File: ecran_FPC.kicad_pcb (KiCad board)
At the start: 4 copper layers, 43 x 43 mm, 24 parts, among them J1 MEC1-110-02-F-D-A, J2 MEC1-110-02-F-D-A, J3 1-2328724-5, SW1 PEC11L-4220K-S0015

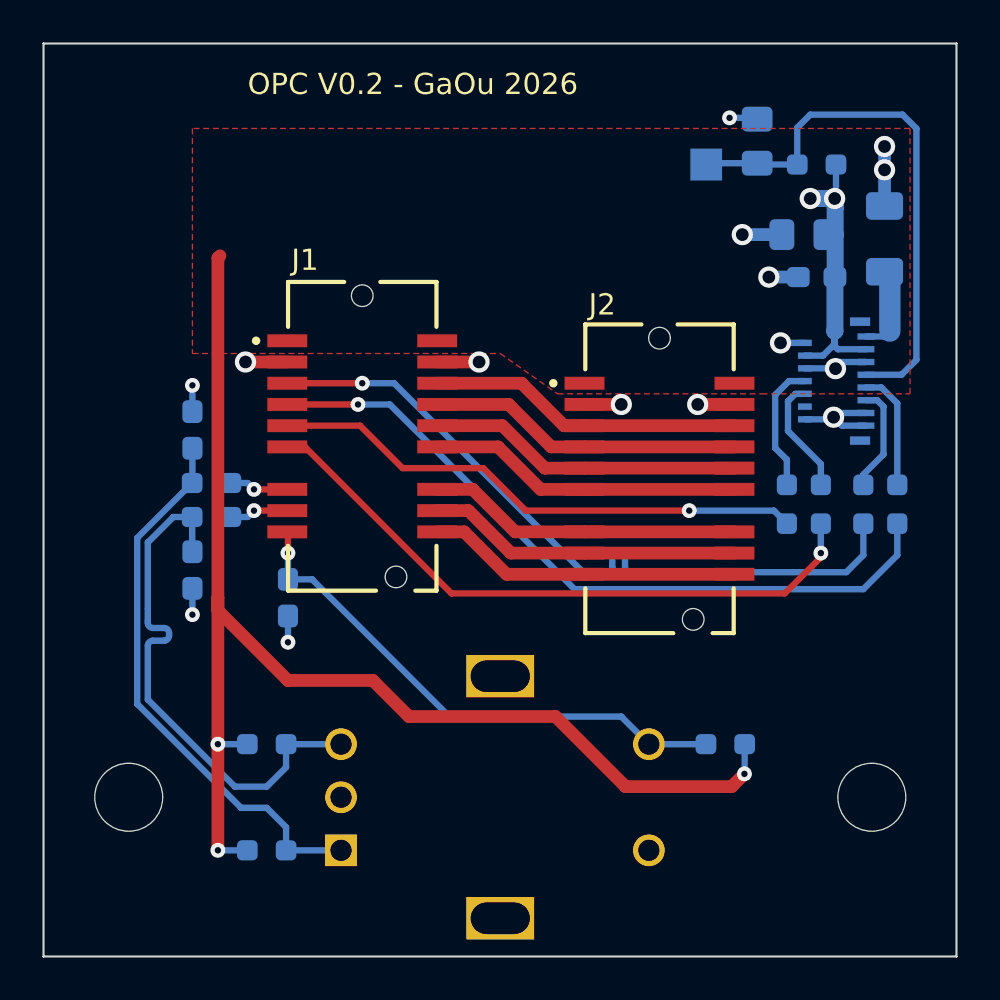
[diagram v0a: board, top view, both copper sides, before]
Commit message: pre prod
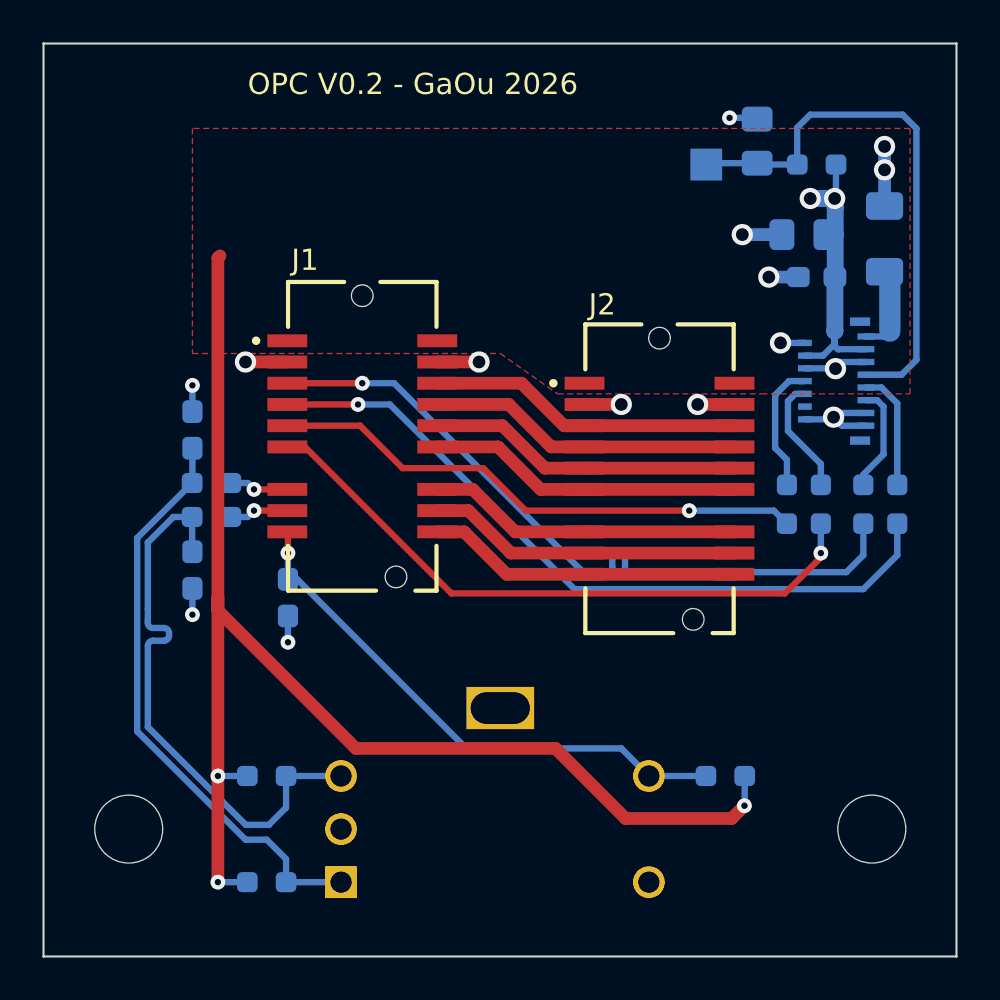
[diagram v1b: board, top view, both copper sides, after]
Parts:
- SW1: value PEC11L-4220K-S0015 -> PEC11L-4220F-S0015
- moved H1 1.50 mm to (104.0, 137.0)
- moved H2 1.50 mm to (139.0, 137.0)
- moved R10 1.50 mm to (110.5, 134.5)
- moved R11 1.50 mm to (110.5, 139.5)
- moved R9 1.50 mm to (132.1, 134.5)
- moved SW1 1.50 mm to (121.5, 137.0)
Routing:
- net +3.3V: track 77.6 -> 79.7 mm
- net Net-(C5-Pad2): track 25.4 -> 27.3 mm
- net Net-(C4-Pad2): track 26.4 -> 27.6 mm
- net /ROTENC_SW: track 25.2 -> 25.8 mm
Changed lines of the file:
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@@
 	(footprint "MountingHole:MountingHole_3.2mm_M3_DIN965"
 		(layer "F.Cu")
-		(at 104 135.5)
+		(at 104 137)
 		(descr "Mounting Hole 3.2mm, M3, no annular, generated by kicad-footprint-generator mountinghole.py")
 		(tags "mountinghole M3 DIN965")
@@
 	(footprint "MountingHole:MountingHole_3.2mm_M3_DIN965"
 		(layer "F.Cu")
-		(at 139 135.5)
+		(at 139 137)
 		(descr "Mounting Hole 3.2mm, M3, no annular, generated by kicad-footprint-generator mountinghole.py")
 		(tags "mountinghole M3 DIN965")
@@
 	(footprint "OPC:PEC11L4220KS0015"
 		(layer "B.Cu")
-		(at 121.5 135.5 90)
+		(at 121.5 137 90)
 		(descr "PEC11L-4220K-S0015-2")
 		(tags "Undefined or Miscellaneous")
 		(property "Reference" "SW1"
-			(at 7.9 0 180)
+			(at 7.9 0 0)
 			(layer "B.SilkS")
 			(effects
@@
 			)
 		)
-		(property "Value" "PEC11L-4220K-S0015"
-			(at 2.5 7.25 90)
+		(property "Value" "PEC11L-4220F-S0015"
+			(at 2.5 7.25 270)
 			(layer "B.SilkS")
 			(hide yes)
@@
 		)
 		(property "Datasheet" ""
-			(at 0 0 90)
+			(at 0 0 270)
 			(layer "B.Fab")
 			(hide yes)
@@
 		)
 		(property "Description" "Rotary encoder, dual channel, incremental quadrate outputs, with switch and MP Pin"
-			(at 0 0 90)
+			(at 0 0 270)
 			(layer "B.Fab")
 			(hide yes)
@@
 			)
 		)
-		(property "MPN" "PEC11L-4220K-S0015 "
+		(property "MPN" "PEC11L-4220F-S0015 "
 			(at 0 0 90)
 			(unlocked yes)
@@
 			)
 		)
-		(property "px_1" "2.13"
+		(property "px_1" "2.35"
 			(at 0 0 90)
 			(unlocked yes)
@@
 			)
 		)
-		(property "px_10" "1.78"
+		(property "px_10" "2.02"
 			(at 0 0 90)
 			(unlocked yes)
@@
 		)
 		(fp_text user "${REFERENCE}"
-			(at 0 -11 90)
+			(at 0 -11 270)
 			(layer "B.Fab")
 			(effects
@@
 		)
 		(pad "MP" thru_hole rect
-			(at -5.7 0)
-			(size 3.2 2)
-			(drill oval 2.8 1.5)
-			(layers "*.Cu" "*.Mask")
-			(remove_unused_layers no)
-			(net "unconnected-(SW1-PadMP)")
-			(pinfunction "MP_MP")
-			(pintype "passive")
-		)
-		(pad "MP" thru_hole rect
 			(at 5.7 0)
 			(size 3.2 2)
@@
 	(footprint "Resistor_SMD:R_0603_1608Metric_Pad0.98x0.95mm_HandSolder"
 		(layer "B.Cu")
-		(at 132.1 133)
+		(at 132.1 134.5)
 		(descr "Resistor SMD 0603 (1608 Metric), square (rectangular) end terminal, IPC-7351 nominal with elongated pad for handsoldering. (Body size source: IPC-SM-782 page 72, https://www.pcb-3d.com/wordpress/wp-content/uploads/ipc-sm-782a_amendment_1_and_2.pdf)")
 		(tags "resistor handsolder")
@@
 	(footprint "Resistor_SMD:R_0603_1608Metric_Pad0.98x0.95mm_HandSolder"
 		(layer "B.Cu")
-		(at 110.5 133)
+		(at 110.5 134.5)
 		(descr "Resistor SMD 0603 (1608 Metric), square (rectangular) end terminal, IPC-7351 nominal with elongated pad for handsoldering. (Body size source: IPC-SM-782 page 72, https://www.pcb-3d.com/wordpress/wp-content/uploads/ipc-sm-782a_amendment_1_and_2.pdf)")
 		(tags "resistor handsolder")
@@
 	(footprint "Resistor_SMD:R_0603_1608Metric_Pad0.98x0.95mm_HandSolder"
 		(layer "B.Cu")
-		(at 110.5 138)
+		(at 110.5 139.5)
 		(descr "Resistor SMD 0603 (1608 Metric), square (rectangular) end terminal, IPC-7351 nominal with elongated pad for handsoldering. (Body size source: IPC-SM-782 page 72, https://www.pcb-3d.com/wordpress/wp-content/uploads/ipc-sm-782a_amendment_1_and_2.pdf)")
 		(tags "resistor handsolder")
@@
 	)
 	(segment
-		(start 117.2 131.7)
-		(end 124.1 131.7)
+		(start 132.4 136.5)
+		(end 133 135.9)
 		(width 0.6)
 		(layer "F.Cu")
@@
 	)
 	(segment
-		(start 127.4 135)
-		(end 132.4 135)
+		(start 108.2 126.7)
+		(end 114.7 133.2)
 		(width 0.6)
 		(layer "F.Cu")
@@
 	)
 	(segment
-		(start 108.2 126.1)
-		(end 108.2 126.7)
+		(start 124.1 133.2)
+		(end 127.4 136.5)
 		(width 0.6)
 		(layer "F.Cu")
@@
 	)
 	(segment
-		(start 111.5 130)
-		(end 115.5 130)
+		(start 114.7 133.2)
+		(end 124.1 133.2)
 		(width 0.6)
 		(layer "F.Cu")
@@
 	)
 	(segment
-		(start 108.2 133)
-		(end 108.2 126.1)
+		(start 127.4 136.5)
+		(end 132.4 136.5)
 		(width 0.6)
 		(layer "F.Cu")
@@
 	)
 	(segment
-		(start 115.5 130)
-		(end 117.2 131.7)
-		(width 0.6)
-		(layer "F.Cu")
-		(net "+3.3V")
-	)
-	(segment
-		(start 132.4 135)
-		(end 133 134.4)
-		(width 0.6)
-		(layer "F.Cu")
-		(net "+3.3V")
-	)
-	(segment
 		(start 108.3 110)
 		(end 108.2 110.1)
@@
 	)
 	(segment
-		(start 124.1 131.7)
-		(end 127.4 135)
+		(start 108.2 139.5)
+		(end 108.2 134.5)
 		(width 0.6)
 		(layer "F.Cu")
@@
 	)
 	(segment
-		(start 108.2 138)
-		(end 108.2 133)
+		(start 108.2 126.1)
+		(end 108.2 126.7)
 		(width 0.6)
 		(layer "F.Cu")
@@
 	)
 	(segment
-		(start 108.2 126.7)
-		(end 111.5 130)
+		(start 108.2 134.5)
+		(end 108.2 126.1)
 		(width 0.6)
 		(layer "F.Cu")
@@
 	)
 	(via
-		(at 108.2 138)
+		(at 108.2 139.5)
 		(size 0.7)
 		(drill 0.3)
@@
 	)
 	(via
-		(at 133 134.4)
+		(at 133 135.9)
 		(size 0.7)
 		(drill 0.3)
@@
 	)
 	(via
-		(at 108.2 133)
+		(at 108.2 134.5)
 		(size 0.7)
 		(drill 0.3)
@@
 	)
 	(segment
-		(start 109.5875 133)
-		(end 108.2 133)
+		(start 109.5875 134.5)
+		(end 108.2 134.5)
 		(width 0.3)
 		(layer "B.Cu")
@@
 	)
 	(segment
-		(start 133.0125 133)
-		(end 133.0125 134.3875)
+		(start 133.0125 134.5)
+		(end 133.0125 135.8875)
 		(width 0.3)
 		(layer "B.Cu")
@@
 	)
 	(segment
-		(start 109.5875 138)
-		(end 108.2 138)
+		(start 109.5875 139.5)
+		(end 108.2 139.5)
 		(width 0.3)
 		(layer "B.Cu")
@@
 	)
 	(segment
-		(start 133.0125 134.3875)
-		(end 133 134.4)
+		(start 133.0125 135.8875)
+		(end 133 135.9)
 		(width 0.3)
 		(layer "B.Cu")
@@
 	)
 	(segment
-		(start 131.1875 133)
-		(end 128.5 133)
+		(start 127.2 133.2)
+		(end 119.9 133.2)
 		(width 0.3)
 		(layer "B.Cu")
@@
 	)
 	(segment
-		(start 119.1 131.7)
-		(end 112.6375 125.2375)
+		(start 128.5 134.5)
+		(end 127.2 133.2)
 		(width 0.3)
 		(layer "B.Cu")
@@
 	)
 	(segment
-		(start 128.5 133)
-		(end 127.2 131.7)
+		(start 131.1875 134.5)
+		(end 128.5 134.5)
 		(width 0.3)
 		(layer "B.Cu")
@@
 	)
 	(segment
-		(start 111.5 125.2375)
-		(end 111.5 124)
+		(start 111.9375 125.2375)
+		(end 111.5 125.2375)
 		(width 0.3)
 		(layer "B.Cu")
@@
 	)
 	(segment
-		(start 127.2 131.7)
-		(end 119.1 131.7)
+		(start 111.5 125.2375)
+		(end 111.5 124)
 		(width 0.3)
 		(layer "B.Cu")
@@
 	)
 	(segment
-		(start 112.6375 125.2375)
-		(end 111.5 125.2375)
+		(start 119.9 133.2)
+		(end 111.9375 125.2375)
 		(width 0.3)
 		(layer "B.Cu")
@@
 	)
 	(segment
-		(start 111.4125 133)
-		(end 114 133)
+		(start 111.4125 134.5)
+		(end 114 134.5)
 		(width 0.3)
 		(layer "B.Cu")
@@
 	)
 	(segment
-		(start 109 135)
-		(end 104.9 130.9)
+		(start 105.9 127.88776)
+		(end 105.9 127.76776)
 		(width 0.3)
 		(layer "B.Cu")
@@
 	)
 	(segment
-		(start 110.5 135)
-		(end 109 135)
+		(start 106.9875 122.3)
+		(end 106.9875 123.925)
 		(width 0.3)
 		(layer "B.Cu")
@@
 	)
 	(segment
-		(start 105.9 127.88776)
-		(end 105.9 127.76776)
+		(start 104.9 132.18995)
+		(end 109.51005 136.8)
 		(width 0.3)
 		(layer "B.Cu")
@@
 	)
 	(segment
-		(start 111.4125 133)
-		(end 111.4125 134.0875)
+		(start 109.51005 136.8)
+		(end 110.6 136.8)
 		(width 0.3)
 		(layer "B.Cu")
@@
 	)
 	(segment
-		(start 106.9875 122.3)
-		(end 106.9875 123.925)
+		(start 110.6 136.8)
+		(end 111.4125 135.9875)
 		(width 0.3)
 		(layer "B.Cu")
@@
 	)
 	(segment
-		(start 111.4125 134.0875)
-		(end 110.5 135)
+		(start 111.4125 135.9875)
+		(end 111.4125 134.5)
 		(width 0.3)
 		(layer "B.Cu")
@@
 	)
 	(segment
-		(start 104.9 130.9)
-		(end 104.9 128.36776)
+		(start 104.9 128.36776)
+		(end 104.9 132.18995)
 		(width 0.3)
 		(layer "B.Cu")
@@
 	)
 	(segment
-		(start 113.8875 137.9)
-		(end 113.9875 138)
-		(width 0.3)
-		(layer "F.Cu")
-		(net "Net-(C4-Pad2)")
-	)
-	(segment
-		(start 111.4125 136.9125)
-		(end 111.4125 138)
+		(start 107 119.0625)
+		(end 107 120.6875)
 		(width 0.3)
 		(layer "B.Cu")
@@
 	)
 	(segment
-		(start 107 119.0625)
-		(end 107 120.6875)
+		(start 107 120.6875)
+		(end 106.9875 120.7)
 		(width 0.3)
 		(layer "B.Cu")
@@
 	)
 	(segment
-		(start 107 120.6875)
-		(end 106.9875 120.7)
+		(start 109.5 137.5)
+		(end 110.5 137.5)
 		(width 0.3)
 		(layer "B.Cu")
@@
 	)
 	(segment
-		(start 109.292893 136)
-		(end 110.5 136)
+		(start 104.4 132.4)
+		(end 109.5 137.5)
 		(width 0.3)
 		(layer "B.Cu")
@@
 	)
 	(segment
-		(start 104.4 123.2875)
-		(end 104.4 131.107107)
+		(start 111.4125 139.5)
+		(end 114 139.5)
 		(width 0.3)
 		(layer "B.Cu")
@@
 	)
 	(segment
-		(start 106.9875 120.7)
-		(end 104.4 123.2875)
+		(start 104.4 123.2875)
+		(end 104.4 132.4)
 		(width 0.3)
 		(layer "B.Cu")
@@
 	)
 	(segment
-		(start 111.4125 138)
-		(end 114 138)
+		(start 111.4125 138.4125)
+		(end 111.4125 139.5)
 		(width 0.3)
 		(layer "B.Cu")
@@
 	)
 	(segment
-		(start 110.5 136)
-		(end 111.4125 136.9125)
+		(start 110.5 137.5)
+		(end 111.4125 138.4125)
 		(width 0.3)
 		(layer "B.Cu")
@@
 	)
 	(segment
-		(start 104.4 131.107107)
-		(end 109.292893 136)
+		(start 106.9875 120.7)
+		(end 104.4 123.2875)
 		(width 0.3)
 		(layer "B.Cu")
